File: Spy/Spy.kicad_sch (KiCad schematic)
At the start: 1 part, among them U1 ESP32-WROOM-E

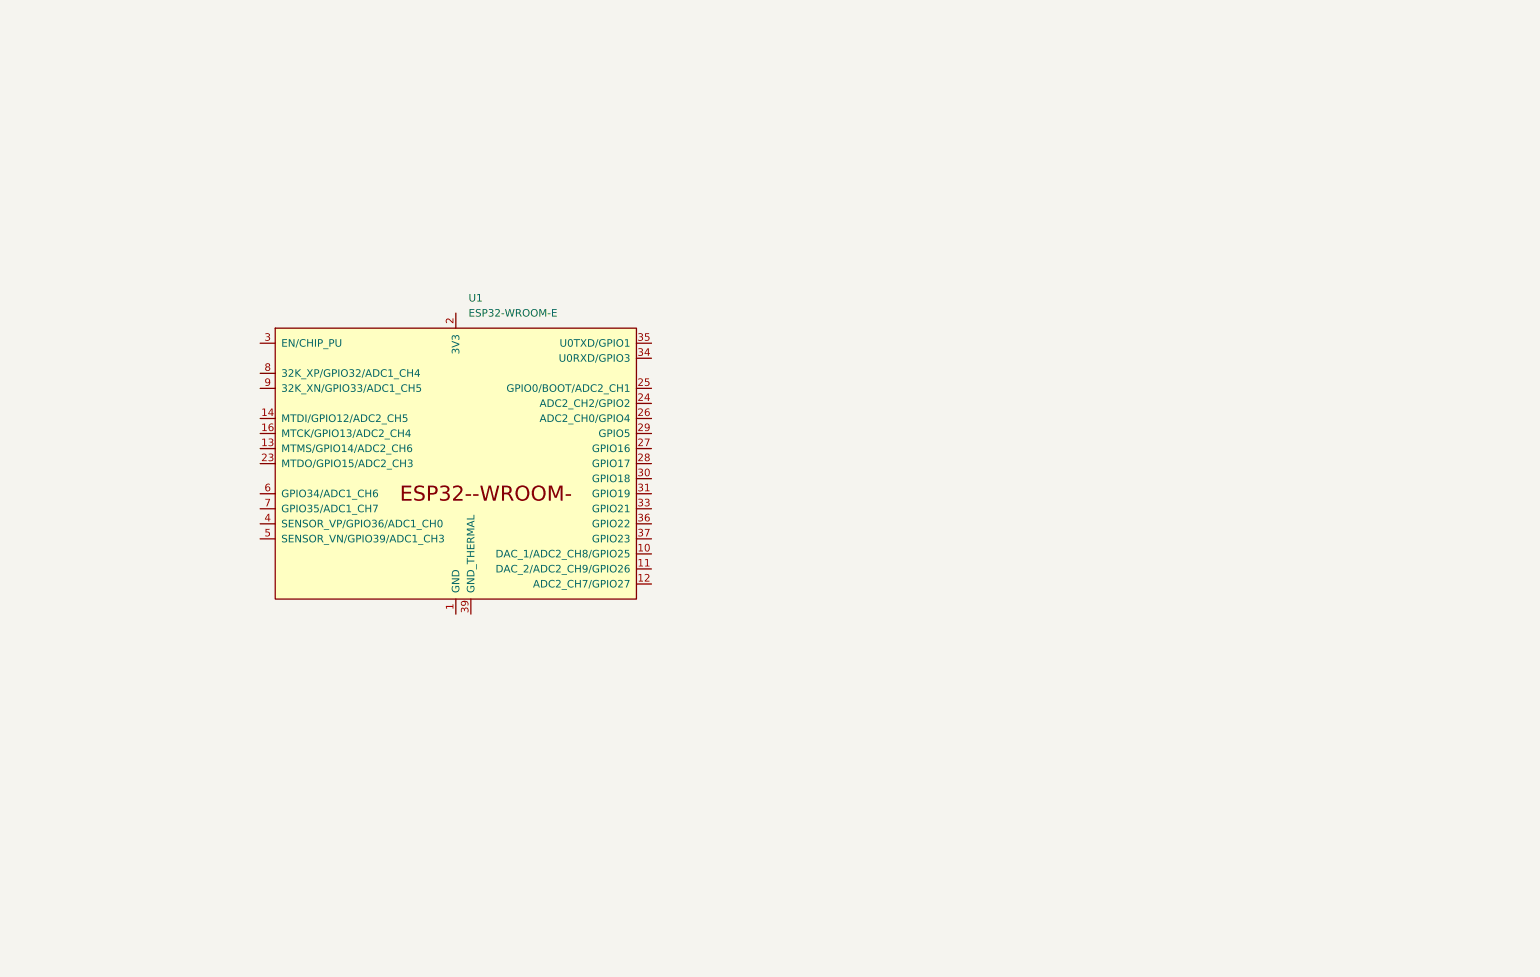
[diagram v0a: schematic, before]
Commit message: kicad libraries
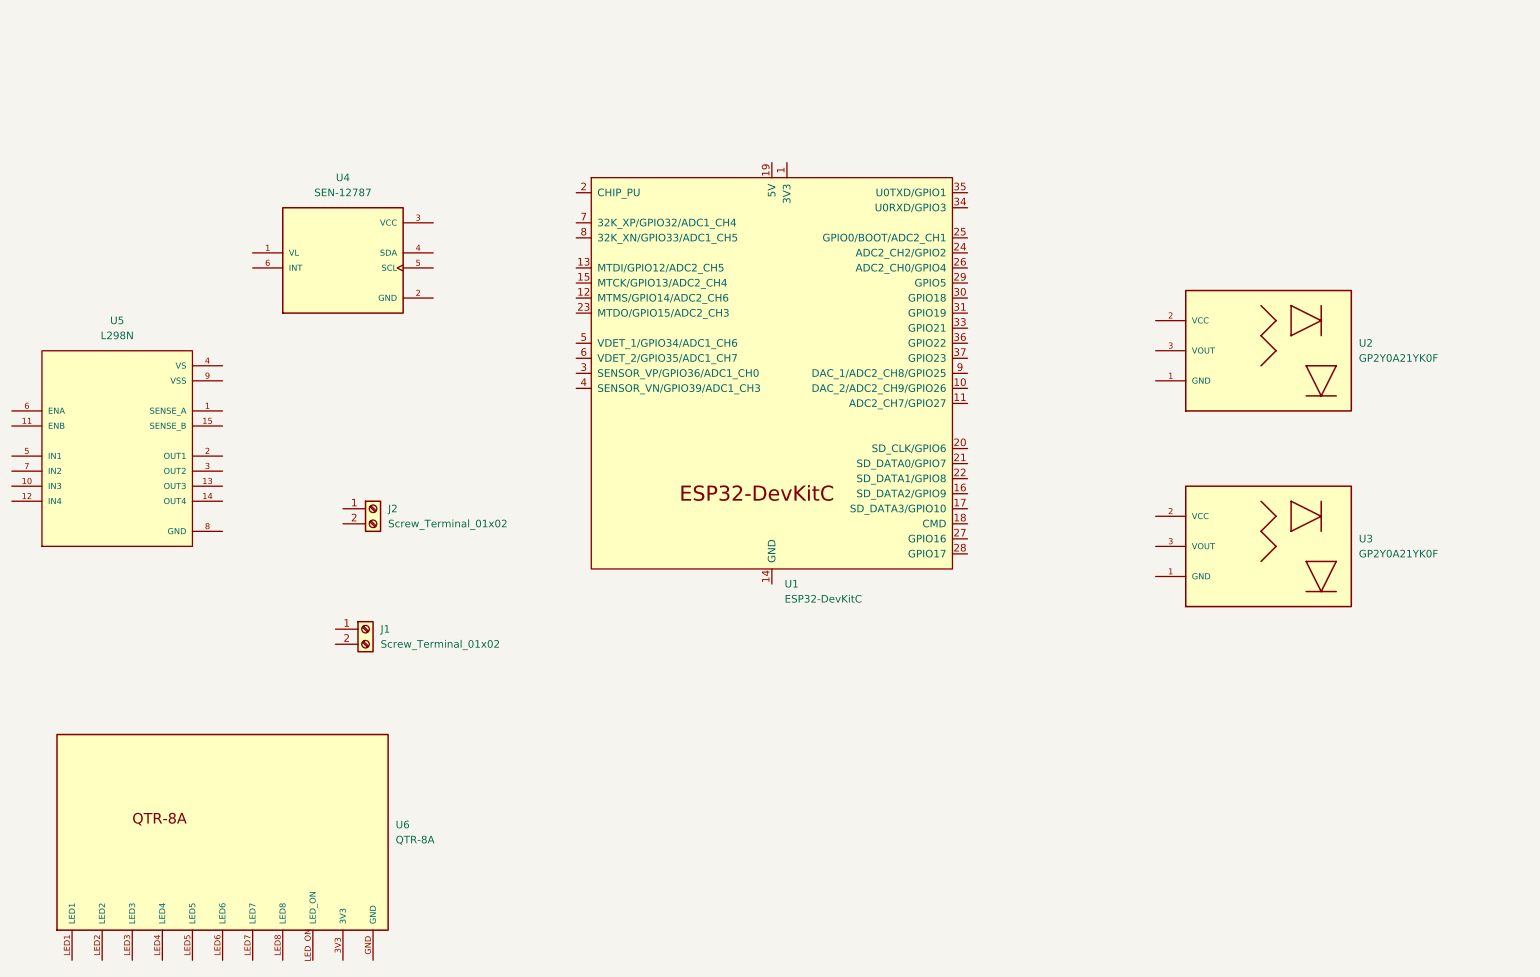
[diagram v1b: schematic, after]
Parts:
- removed U1: ESP32-WROOM-E, PCM_Espressif:ESP32-WROOM-32E, symbol Espressif:ESP32-WROOM-E
- added J1, J2: Screw_Terminal_01x02, Connector_Phoenix_MSTB:PhoenixContact_MSTBA_2,5_2-G_1x02_P5.00mm_Horizontal, symbol Connector:Screw_Terminal_01x02
- added U1: ESP32-DevKitC, PCM_Espressif:ESP32-DevKitC, symbol Espressif:ESP32-DevKitC
- added U2, U3: GP2Y0A21YK0F, GP2Y0A21YK0F:22-23-2031, symbol GP2Y0A21YK0F:GP2Y0A21YK0F
- added U4: SEN-12787, SEN-12787:MODULE_SEN-12787, symbol SEN-12787:SEN-12787
- added U5: L298N, L298N:TO127P2020X500X2100-15, symbol L298N:L298N
- added U6: QTR-8A, QTR-8A:QTR-8A, symbol QTR-8A:QTR-8A
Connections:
- new net: U1.14 (GND), U1.32 (GND), U1.38 (GND)

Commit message: schematic (1) :D
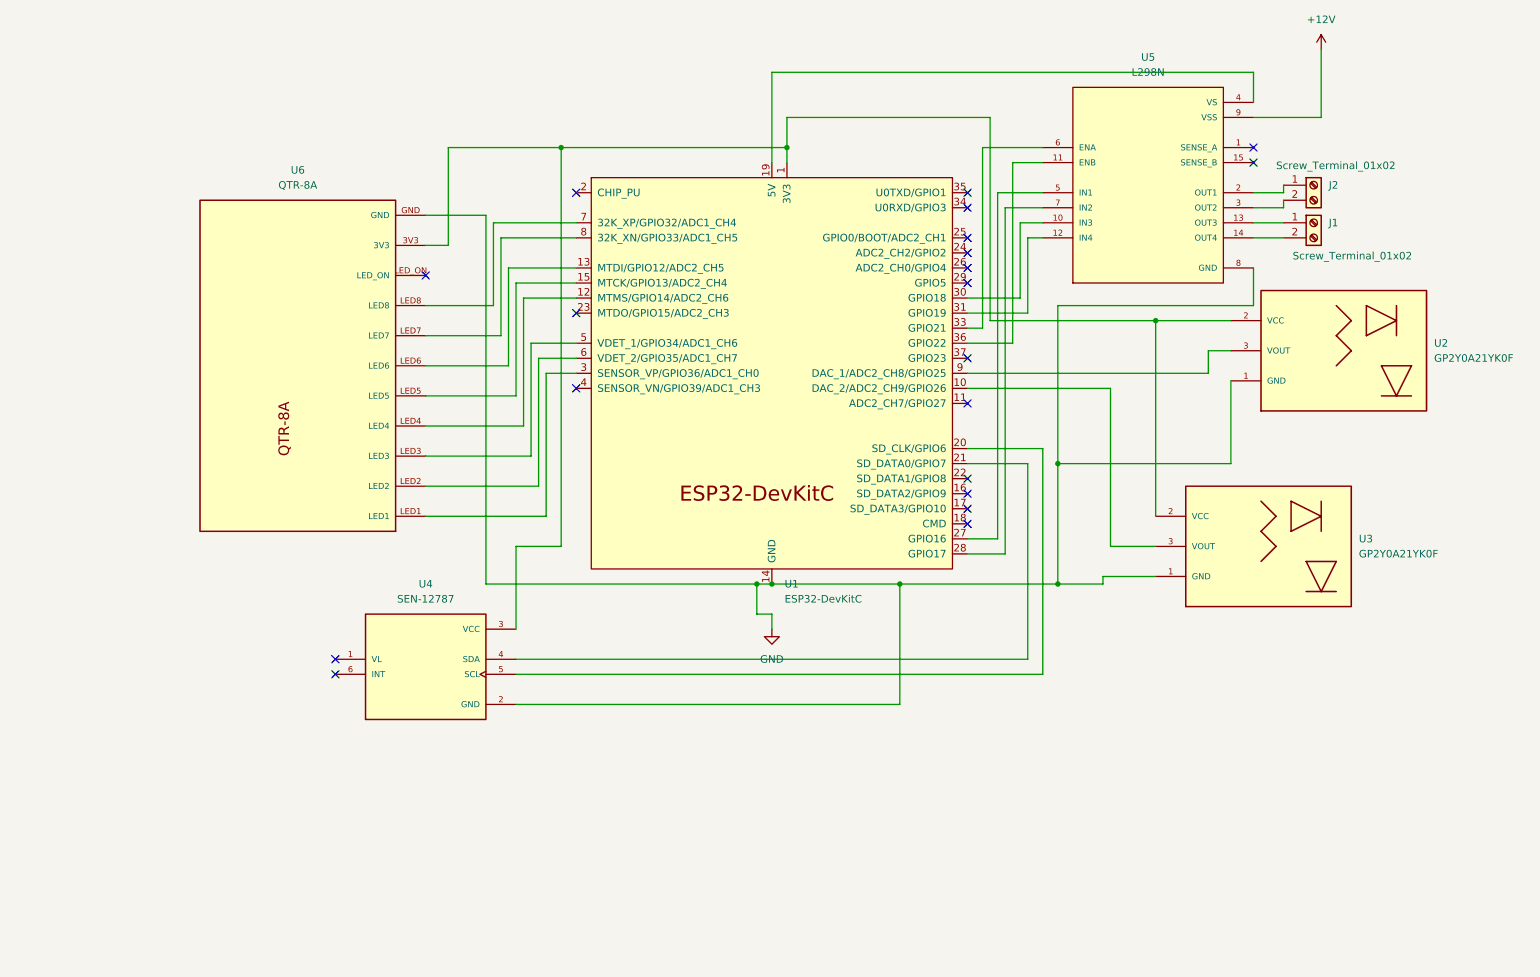
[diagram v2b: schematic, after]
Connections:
- net at U1.1 (3V3): now also U2.2 (VCC), U3.2 (VCC), U4.3 (VCC), U6.3V3
- net at U1.10 (DAC_2/ADC2_CH9/GPIO26): now also U3.3 (VOUT)
- net at U1.12 (MTMS/GPIO14/ADC2_CH6): now also U6.LED4
- net at U1.13 (MTDI/GPIO12/ADC2_CH5): now also U6.LED6
- net GND: now reaches U1.14 (GND), U1.32 (GND), U1.38 (GND)
- net GND: now also U2.1 (GND), U3.1 (GND), U4.2 (GND), U5.8 (GND), U6.GND
- net at U1.15 (MTCK/GPIO13/ADC2_CH4): now also U6.LED5
- net at U1.19 (5V): now also U5.4 (VS)
- net at U1.20 (SD_CLK/GPIO6): now also U4.5 (SCL)
- net at U1.21 (SD_DATA0/GPIO7): now also U4.4 (SDA)
- net at U1.27 (GPIO16): now also U5.5 (IN1)
- net at U1.28 (GPIO17): now also U5.7 (IN2)
- net at U1.3 (SENSOR_VP/GPIO36/ADC1_CH0): now also U6.LED1
- net at U1.30 (GPIO18): now also U5.10 (IN3)
- net at U1.31 (GPIO19): now also U5.12 (IN4)
- net at U1.33 (GPIO21): now also U5.6 (ENA)
- net at U1.36 (GPIO22): now also U5.11 (ENB)
- net at U1.5 (VDET_1/GPIO34/ADC1_CH6): now also U6.LED3
- net at U1.6 (VDET_2/GPIO35/ADC1_CH7): now also U6.LED2
- net at U1.7 (32K_XP/GPIO32/ADC1_CH4): now also U6.LED8
- net at U1.8 (32K_XN/GPIO33/ADC1_CH5): now also U6.LED7
- net at U1.9 (DAC_1/ADC2_CH8/GPIO25): now also U2.3 (VOUT)
- net at J1.1 (Pin_1): now also U5.13 (OUT3)
- net at J1.2 (Pin_2): now also U5.14 (OUT4)
- net at J2.1 (Pin_1): now also U5.2 (OUT1)
- net at J2.2 (Pin_2): now also U5.3 (OUT2)
- net +12V: now reaches U5.9 (VSS)
- no-connect marks 0 -> 20
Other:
- moved on the sheet: J1, J2, U2, U4, U5, U6
